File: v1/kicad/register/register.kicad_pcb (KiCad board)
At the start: 2 copper layers, 73 x 46 mm, 5 parts, among them J1 DBUS, J2 BASE, J3 CTRL, U1 74LS173, U2 74LS173

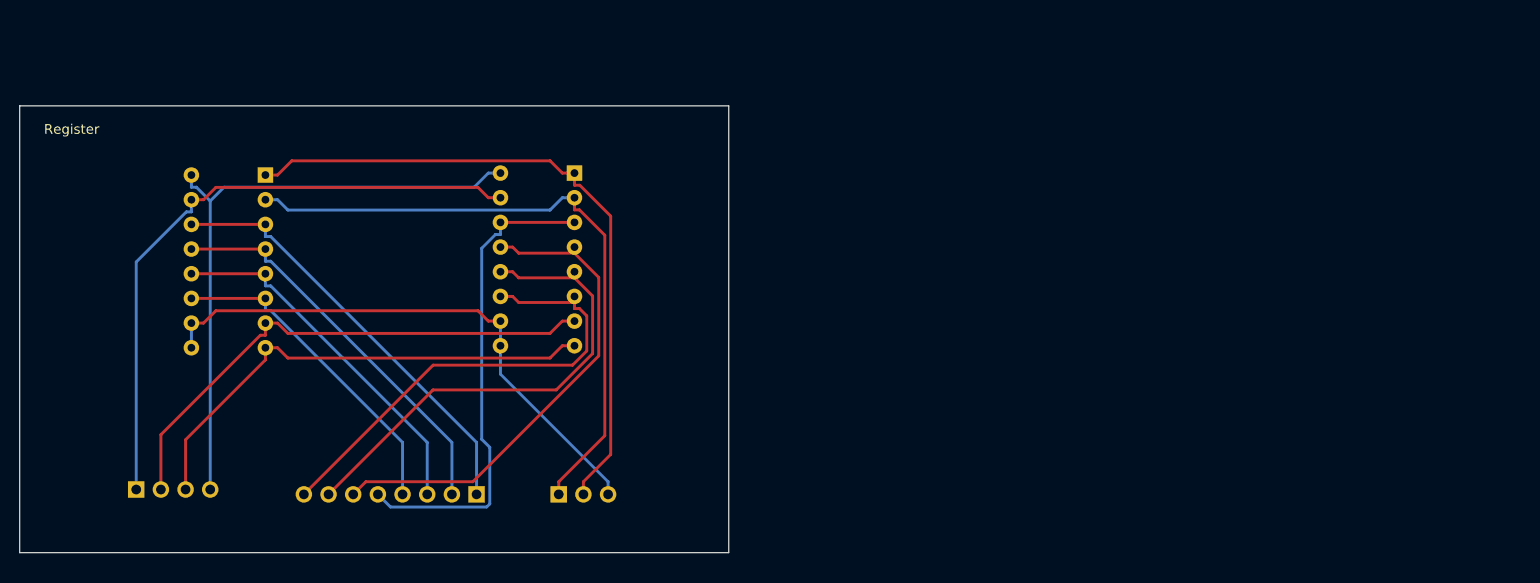
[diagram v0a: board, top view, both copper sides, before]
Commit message: progress on kicad implementation
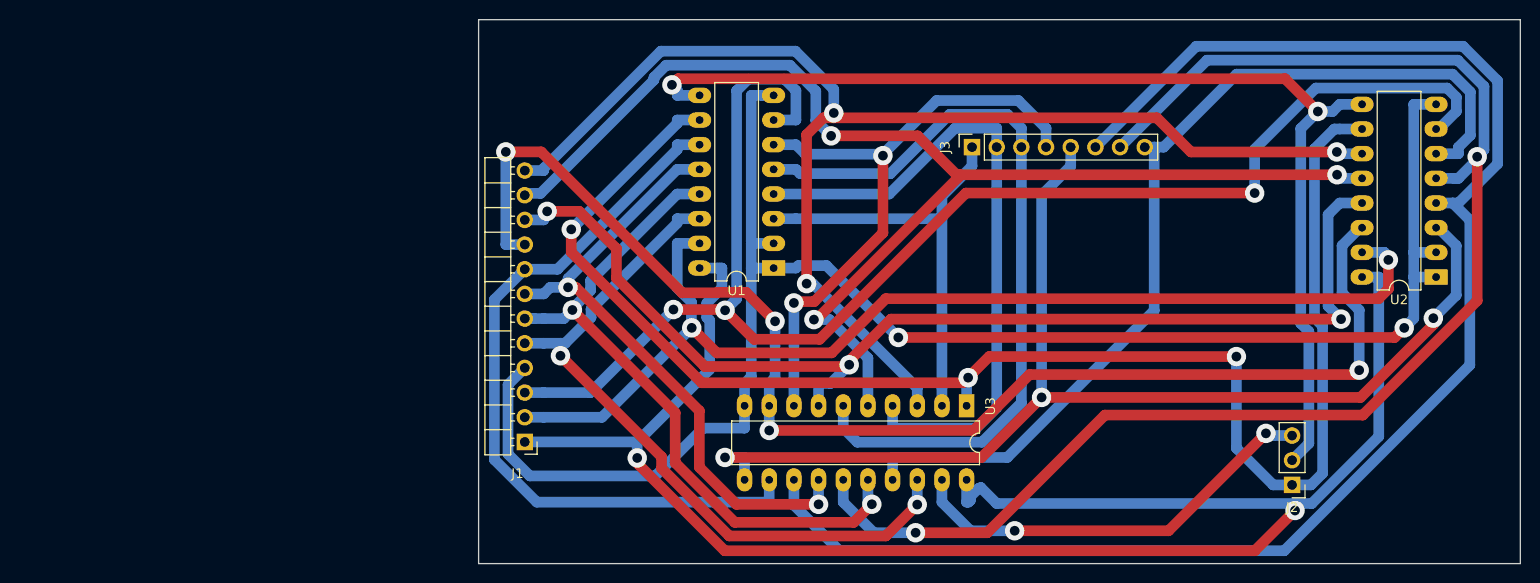
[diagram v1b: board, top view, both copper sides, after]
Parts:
- added U3: 74LS244, Package_DIP:DIP-20_W7.62mm_LongPads, F.Cu at (141.5, 104.4)
- J1: value DBUS -> RegisterSocket (active-high reset); footprint Connector_PinSocket_2.54mm:PinSocket_1x08_P2.54mm_Vertical -> LNCPU:RegisterPort; moved to F.Cu
- J2: value BASE -> RegisterCtrl; footprint Connector_PinSocket_2.54mm:PinSocket_1x04_P2.54mm_Vertical -> Connector_PinHeader_2.54mm:PinHeader_1x03_P2.54mm_Vertical; moved to F.Cu
- J3: value CTRL -> ASYNC_{out}; footprint Connector_PinHeader_2.54mm:PinHeader_1x03_P2.54mm_Vertical -> Connector_PinSocket_2.54mm:PinSocket_1x08_P2.54mm_Vertical; moved to F.Cu
- U1, U2: value 74LS173 -> 74HC173; footprint Package_DIP:DIP-16_W7.62mm -> Package_DIP:DIP-16_W7.62mm_LongPads; moved to F.Cu
- moved J2 119.0 mm to (175.0, 112.5), turned to 180 degrees
- moved U2 89.3 mm to (189.8, 91.1)
- moved J3 55.6 mm to (142.1, 77.8), turned to 90 degrees
- moved U1 53.2 mm to (121.6, 90.2)
- moved J1 7.33 mm to (96.0, 108.1), turned to 180 degrees
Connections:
- J1 pad 1: Net-(J1-Pin_1) -> Net-(J1-VCC)
- J1 pad 2: Net-(J1-Pin_2) -> Net-(J1-RST)
- J1 pad 3: Net-(J1-Pin_3) -> Net-(J1-CLK)
- J1 pad 4: Net-(J1-Pin_4) -> Net-(J1-GND)
- J1 pad 5: Net-(J1-Pin_5) -> /DBUS0
- J1 pad 6: Net-(J1-Pin_6) -> /DBUS1
- J1 pad 7: Net-(J1-Pin_7) -> /DBUS2
- J1 pad 8: Net-(J1-Pin_8) -> /DBUS3
- J2 pad 1: Net-(J2-Pin_1) -> Net-(J2-~{EN})
- J2 pad 2: Net-(J2-Pin_2) -> Net-(J2-~{R_{in}})
- J2 pad 3: Net-(J2-Pin_3) -> Net-(J2-~{R_{out}})
- J3 pad 1: Net-(J3-Pin_1) -> /ASYNC0
- J3 pad 2: Net-(J3-Pin_2) -> /ASYNC1
- J3 pad 3: Net-(J3-Pin_3) -> /ASYNC2
- U1 pad 1: Net-(J3-Pin_2) -> Net-(J1-GND)
- U1 pad 10: Net-(J3-Pin_3) -> Net-(J2-~{EN})
- U1 pad 11: Net-(J1-Pin_4) -> /DBUS3
- U1 pad 12: Net-(J1-Pin_3) -> /DBUS2
- U1 pad 13: Net-(J1-Pin_2) -> /DBUS1
- U1 pad 14: Net-(J1-Pin_1) -> /DBUS0
- U1 pad 15: Net-(J2-Pin_1) -> Net-(J1-RST)
- U1 pad 16: Net-(J2-Pin_4) -> Net-(J1-VCC)
- U1 pad 2: Net-(J3-Pin_1) -> Net-(J1-GND)
- U1 pad 3: Net-(J1-Pin_1) -> /ASYNC0
- U1 pad 4: Net-(J1-Pin_2) -> /ASYNC1
- U1 pad 5: Net-(J1-Pin_3) -> /ASYNC2
- U1 pad 6: Net-(J1-Pin_4) -> /ASYNC3
- U1 pad 7: Net-(J2-Pin_2) -> Net-(J1-CLK)
- U1 pad 8: Net-(J2-Pin_3) -> Net-(J1-GND)
- U1 pad 9: Net-(J3-Pin_3) -> Net-(J2-~{R_{in}})
- U2 pad 1: Net-(J3-Pin_2) -> Net-(J1-GND)
- U2 pad 10: Net-(J3-Pin_3) -> Net-(J2-~{EN})
- U2 pad 11: Net-(J1-Pin_8) -> /DBUS7
- U2 pad 12: Net-(J1-Pin_7) -> /DBUS6
- U2 pad 13: Net-(J1-Pin_6) -> /DBUS5
- U2 pad 14: Net-(J1-Pin_5) -> /DBUS4
- U2 pad 15: Net-(J2-Pin_1) -> Net-(J1-RST)
- U2 pad 16: Net-(J2-Pin_4) -> Net-(J1-VCC)
- U2 pad 2: Net-(J3-Pin_1) -> Net-(J1-GND)
- U2 pad 3: Net-(J1-Pin_5) -> /ASYNC4
- U2 pad 4: Net-(J1-Pin_6) -> /ASYNC5
- U2 pad 5: Net-(J1-Pin_7) -> /ASYNC6
- U2 pad 6: Net-(J1-Pin_8) -> /ASYNC7
- U2 pad 7: Net-(J2-Pin_2) -> Net-(J1-CLK)
- U2 pad 8: Net-(J2-Pin_3) -> Net-(J1-GND)
- U2 pad 9: Net-(J3-Pin_3) -> Net-(J2-~{R_{in}})
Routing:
- net Net-(J1-VCC): track 0.00 -> 179.0 mm, vias 0 -> 2
- net Net-(J1-GND): track 0.00 -> 177.3 mm, vias 0 -> 2
- net /ASYNC5: track 0.00 -> 163.2 mm
- net Net-(J2-~{EN}): track 0.00 -> 158.4 mm, vias 0 -> 3
- net Net-(J1-CLK): track 0.00 -> 154.3 mm, vias 0 -> 3
- net /ASYNC6: track 0.00 -> 148.7 mm, vias 0 -> 2
- net /DBUS4: track 0.00 -> 137.7 mm, vias 0 -> 4
- net /DBUS7: track 0.00 -> 134.0 mm, vias 0 -> 3
- net /DBUS6: track 0.00 -> 131.9 mm, vias 0 -> 3
- net /ASYNC4: track 0.00 -> 121.9 mm, vias 0 -> 3
- net /DBUS5: track 0.00 -> 117.0 mm, vias 0 -> 3
- net Net-(J1-RST): track 0.00 -> 114.4 mm, vias 0 -> 2
- net Net-(J2-~{R_{in}}): track 0.00 -> 114.3 mm, vias 0 -> 2
- net /ASYNC7: track 0.00 -> 98.9 mm
- net /ASYNC2: track 0.00 -> 80.0 mm
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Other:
- board size 73 x 46 mm -> 107.2 x 56 mm
- board text removed: "Register"
